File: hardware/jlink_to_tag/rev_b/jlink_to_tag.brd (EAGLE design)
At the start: 29.2 x 35.6 mm, 12 parts, among them J2 JLINK_6PIN_TAG-CON, U1 LT1763CS8-3.3

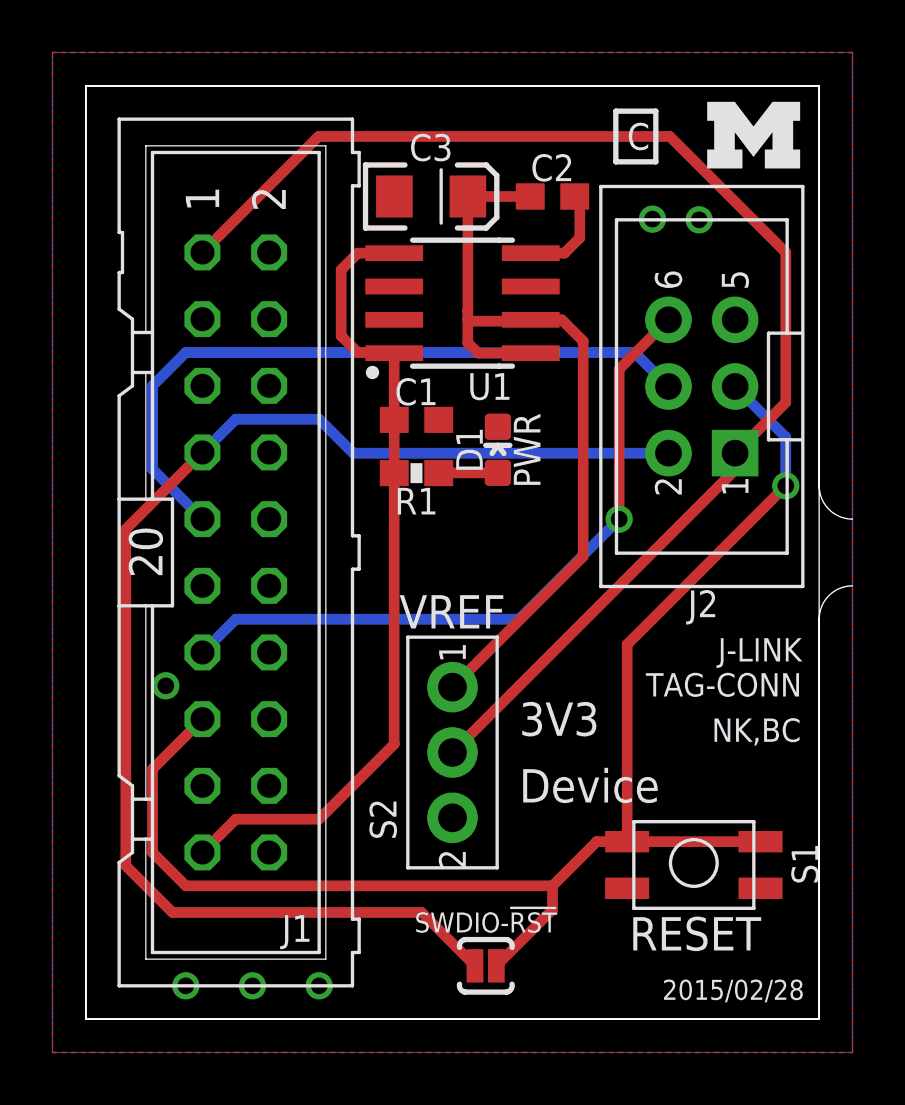
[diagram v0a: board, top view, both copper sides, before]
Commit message: revert rev b to the version that was fabbed
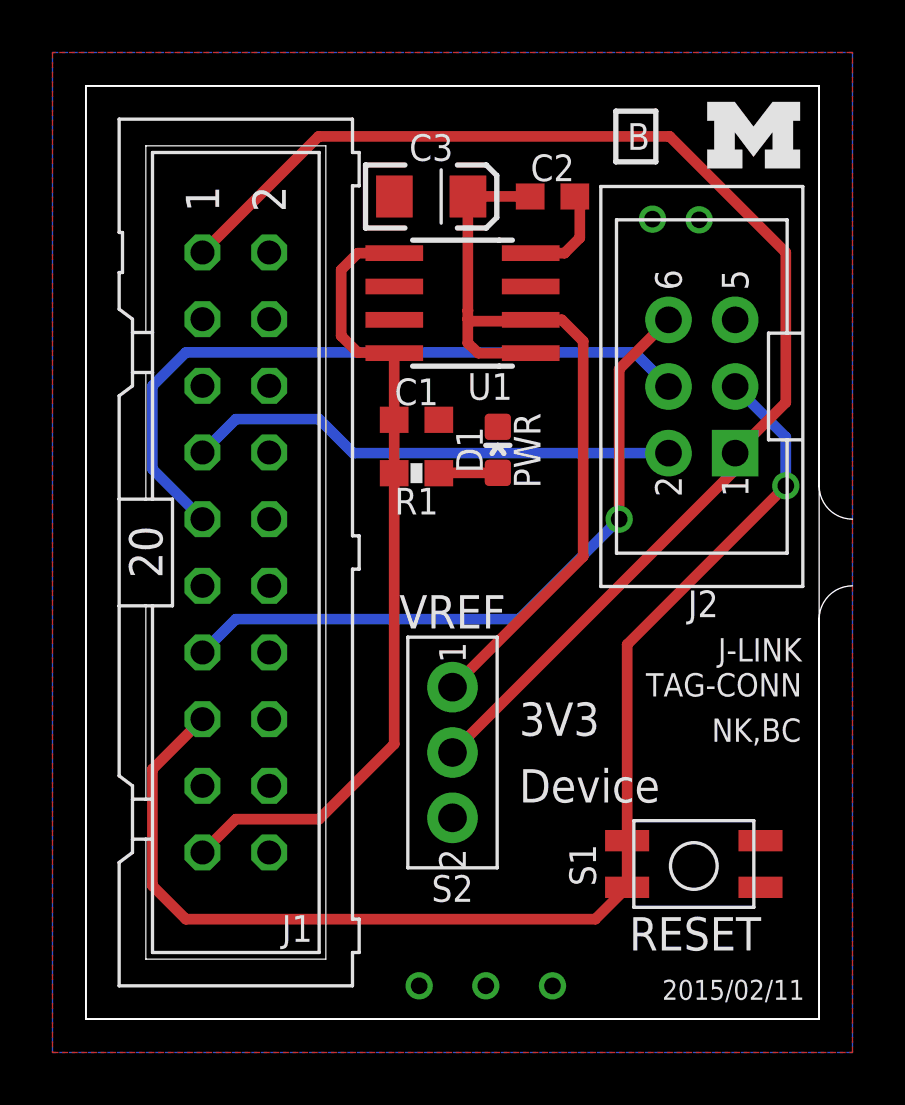
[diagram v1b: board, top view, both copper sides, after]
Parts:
- removed SJ1: SOLDERJUMPERNC2, SparkFun-Passives:SJ_2S-NOTRACE
- turned S1 to 0 degrees
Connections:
- net GND: now also S1.P$3; no longer S1.P$2
- net NRESET: now also S1.P$2; no longer S1.P$3, SJ1.1
- net SWDIO/TMS: no longer SJ1.2
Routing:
- net SWDIO/TMS: track 50.7 -> 18.8 mm
- net NRESET: track 54.8 -> 48.6 mm
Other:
- board text added: "2015/02/11"
- board text added: "B"
- board text removed: "2015/02/28"
- board text removed: "C"
- board text removed: "SWDIO-!RST"
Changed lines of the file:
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@@
 <setting verticaltext="up"/>
 </settings>
-<grid distance="10" unitdist="mil" unit="mil" style="lines" multiple="1" display="yes" altdistance="0.005" altunitdist="inch" altunit="inch"/>
+<grid distance="0.05" unitdist="inch" unit="inch" style="lines" multiple="1" display="yes" altdistance="0.005" altunitdist="inch" altunit="inch"/>
 <layers>
 <layer number="1" name="Top" color="4" fill="1" visible="yes" active="yes"/>
@@
 TAG-CONN</text>
 <text x="27.2542" y="10.5664" size="0.889" layer="21" font="vector" ratio="12" align="bottom-right">NK,BC</text>
-<text x="27.3812" y="0.7366" size="0.762" layer="21" font="vector" ratio="12" align="bottom-right">2015/02/28</text>
+<text x="27.3812" y="0.7366" size="0.762" layer="21" font="vector" ratio="12" align="bottom-right">2015/02/11</text>
 <text x="16.3068" y="21.6662" size="1.016" layer="21" ratio="12" rot="R90" align="top-center">PWR</text>
 <wire x1="0" y1="35.56" x2="0" y2="20.32" width="0" layer="151"/>
@@
 <text x="16.51" y="8.89" size="1.27" layer="21" font="vector" ratio="12" align="center-left">Device</text>
 <text x="13.97" y="14.8844" size="1.27" layer="21" font="vector" ratio="12" rot="R180" align="top-center">VREF</text>
-<text x="21.0566" y="33.6296" size="1.016" layer="21" font="vector" ratio="12" align="center">C</text>
+<text x="21.0566" y="33.6296" size="1.016" layer="21" font="vector" ratio="12" align="center">B</text>
 <wire x1="20.193" y1="32.6644" x2="21.717" y2="32.6644" width="0.2032" layer="21"/>
 <wire x1="21.717" y1="32.6644" x2="21.717" y2="34.5948" width="0.2032" layer="21"/>
 <wire x1="21.717" y1="34.5948" x2="20.193" y2="34.5948" width="0.2032" layer="21"/>
 <wire x1="20.193" y1="34.5948" x2="20.193" y2="32.6644" width="0.2032" layer="21"/>
-<text x="15.24" y="3.302" size="0.762" layer="21" font="vector" ratio="12" align="bottom-center">SWDIO-!RST</text>
-<circle x="10.922" y="24.638" radius="0.254" width="0" layer="21"/>
 </plain>
 <attributes>
@@
 <attribute name="VALUE" x="11.5824" y="19.6596" size="0.4064" layer="27" font="vector"/>
 </element>
-<element name="S1" library="switches" package="EVQP2" value="EVQP2" x="23.1648" y="5.8928" smashed="yes" rot="R180">
-<attribute name="DIGIKEY" value="P11084SCT-ND" x="23.1648" y="5.8928" size="1.778" layer="27" rot="R180" display="off"/>
-<attribute name="NAME" x="26.8922" y="5.9182" size="1.016" layer="25" font="vector" ratio="12" rot="R270" align="bottom-center"/>
-<attribute name="VALUE" x="26.4668" y="9.0488" size="1.27" layer="27" font="vector" ratio="10" rot="R180"/>
+<element name="S1" library="switches" package="EVQP2" value="EVQP2" x="23.1648" y="5.8928" smashed="yes">
+<attribute name="DIGIKEY" value="P11084SCT-ND" x="23.1648" y="5.8928" size="1.778" layer="27" display="off"/>
+<attribute name="NAME" x="19.4374" y="5.8674" size="1.016" layer="25" font="vector" ratio="12" rot="R90" align="bottom-center"/>
+<attribute name="VALUE" x="19.8628" y="2.7368" size="1.27" layer="27" font="vector" ratio="10"/>
 </element>
 <element name="S2" library="switches" package="TE_SSA12/SPDT" value="TE_SSA12/SPDT" x="13.97" y="10.16" smashed="yes" rot="R270">
 <attribute name="DIGIKEY" value="450-1602-ND" x="13.97" y="10.16" size="1.778" layer="27" rot="R270" display="off"/>
-<attribute name="NAME" x="11.8364" y="7.62" size="1.016" layer="25" font="vector" ratio="12" rot="R90" align="bottom-center"/>
+<attribute name="NAME" x="13.97" y="5.4864" size="1.016" layer="25" font="vector" ratio="12" rot="R180" align="bottom-center"/>
 <attribute name="VALUE" x="10.795" y="10.16" size="1.016" layer="27" font="vector" ratio="12" rot="R270" align="bottom-center"/>
-</element>
-<element name="SJ1" library="SparkFun-Passives" package="SJ_2S-NOTRACE" value="SOLDERJUMPERNC2" x="15.24" y="2.032" smashed="yes" rot="R180">
-<attribute name="VALUE" x="16.1925" y="3.683" size="0.4064" layer="27" rot="R180"/>
 </element>
 </elements>
@@
 <vertex x="-1.27" y="-1.27"/>
 </polygon>
-<contactref element="S1" pad="P$2"/>
+<contactref element="S1" pad="P$3"/>
 <contactref element="S1" pad="P$4"/>
-<via x="3.81" y="1.27" extent="1-16" drill="0.635"/>
-<via x="6.35" y="1.27" extent="1-16" drill="0.635"/>
-<via x="8.89" y="1.27" extent="1-16" drill="0.635"/>
+<via x="12.7" y="1.27" extent="1-16" drill="0.635"/>
+<via x="15.24" y="1.27" extent="1-16" drill="0.635"/>
+<via x="17.78" y="1.27" extent="1-16" drill="0.635"/>
 <via x="21.59" y="30.48" extent="1-16" drill="0.635"/>
 <via x="23.368" y="30.4546" extent="1-16" drill="0.635"/>
-<via x="3.048" y="12.7" extent="1-16" drill="0.635"/>
 </signal>
 <signal name="NRESET">
@@
 <contactref element="J2" pad="3"/>
 <contactref element="S1" pad="P$1"/>
-<contactref element="S1" pad="P$3"/>
+<contactref element="S1" pad="P$2"/>
 <wire x1="4.445" y1="11.43" x2="2.54" y2="9.525" width="0.4064" layer="1"/>
-<wire x1="25.7048" y1="6.7628" x2="20.6248" y2="6.7628" width="0.4064" layer="1"/>
+<wire x1="2.54" y1="9.525" x2="2.54" y2="5.08" width="0.4064" layer="1"/>
+<wire x1="2.54" y1="5.08" x2="3.81" y2="3.81" width="0.4064" layer="1"/>
+<wire x1="20.6248" y1="5.0228" x2="20.6248" y2="6.8008" width="0.4064" layer="1"/>
 <via x="26.67" y="20.32" extent="1-16" drill="0.635"/>
 <wire x1="26.67" y1="20.32" x2="26.67" y2="22.1742" width="0.4064" layer="16"/>
 <wire x1="26.67" y1="22.1742" x2="24.7396" y2="24.1046" width="0.4064" layer="16"/>
-<wire x1="20.6248" y1="6.7628" x2="20.6248" y2="14.2748" width="0.4064" layer="1"/>
+<wire x1="3.81" y1="3.81" x2="19.412" y2="3.81" width="0.4064" layer="1"/>
+<wire x1="19.412" y1="3.81" x2="20.6248" y2="5.0228" width="0.4064" layer="1"/>
+<wire x1="20.6248" y1="6.8008" x2="20.6248" y2="14.2748" width="0.4064" layer="1"/>
 <wire x1="20.6248" y1="14.2748" x2="26.67" y2="20.32" width="0.4064" layer="1"/>
-<contactref element="SJ1" pad="1"/>
-<wire x1="2.54" y1="9.525" x2="2.54" y2="6.35" width="0.4064" layer="1"/>
-<wire x1="2.54" y1="6.35" x2="3.81" y2="5.08" width="0.4064" layer="1"/>
-<wire x1="3.81" y1="5.08" x2="17.78" y2="5.08" width="0.4064" layer="1"/>
-<wire x1="17.78" y1="5.08" x2="19.4628" y2="6.7628" width="0.4064" layer="1"/>
-<wire x1="19.4628" y1="6.7628" x2="20.6248" y2="6.7628" width="0.4064" layer="1"/>
-<wire x1="15.6409" y1="2.032" x2="17.78" y2="4.1711" width="0.4064" layer="1"/>
-<wire x1="17.78" y1="4.1711" x2="17.78" y2="5.08" width="0.4064" layer="1"/>
 </signal>
 <signal name="SWCLK/TCK">
@@
 <wire x1="5.715" y1="22.86" x2="8.89" y2="22.86" width="0.4064" layer="16"/>
 <wire x1="8.89" y1="22.86" x2="10.1854" y2="21.5646" width="0.4064" layer="16"/>
-<contactref element="SJ1" pad="2"/>
-<wire x1="4.445" y1="21.59" x2="1.524" y2="18.669" width="0.4064" layer="1"/>
-<wire x1="1.524" y1="18.669" x2="1.524" y2="5.842" width="0.4064" layer="1"/>
-<wire x1="1.524" y1="5.842" x2="3.302" y2="4.064" width="0.4064" layer="1"/>
-<wire x1="3.302" y1="4.064" x2="12.7953" y2="4.064" width="0.4064" layer="1"/>
-<wire x1="12.7953" y1="4.064" x2="14.8273" y2="2.032" width="0.4064" layer="1"/>
 </signal>
 <signal name="SWO/TDO">

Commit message: bug fixes to rev b
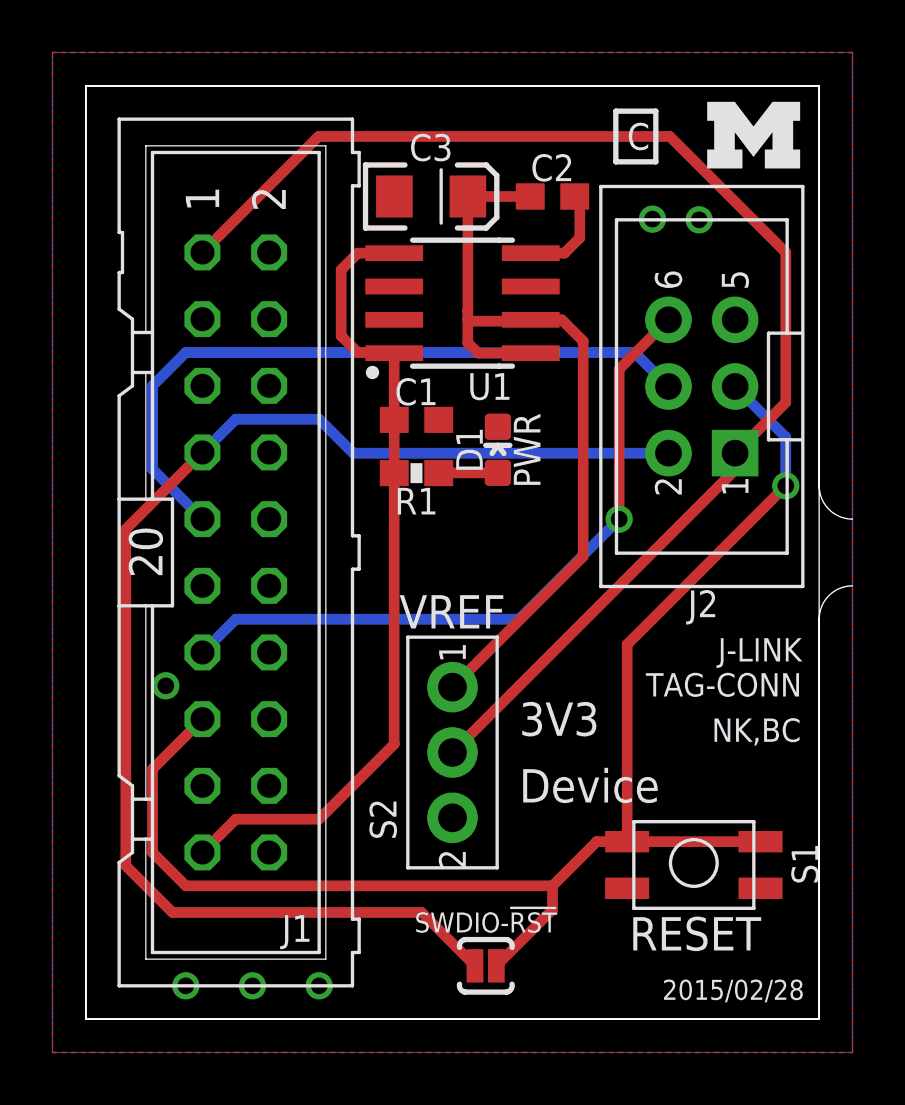
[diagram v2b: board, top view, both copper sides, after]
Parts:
- added SJ1: SOLDERJUMPERNC2, SparkFun-Passives:SJ_2S-NOTRACE
- turned S1 to 180 degrees
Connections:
- net GND: now also S1.P$2; no longer S1.P$3
- net NRESET: now also S1.P$3, SJ1.1; no longer S1.P$2
- net SWDIO/TMS: now also SJ1.2
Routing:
- net SWDIO/TMS: track 18.8 -> 50.7 mm
- net NRESET: track 48.6 -> 54.8 mm
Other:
- board text added: "2015/02/28"
- board text added: "C"
- board text added: "SWDIO-!RST"
- board text removed: "2015/02/11"
- board text removed: "B"
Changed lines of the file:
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@@
 <setting verticaltext="up"/>
 </settings>
-<grid distance="0.05" unitdist="inch" unit="inch" style="lines" multiple="1" display="yes" altdistance="0.005" altunitdist="inch" altunit="inch"/>
+<grid distance="10" unitdist="mil" unit="mil" style="lines" multiple="1" display="yes" altdistance="0.005" altunitdist="inch" altunit="inch"/>
 <layers>
 <layer number="1" name="Top" color="4" fill="1" visible="yes" active="yes"/>
@@
 TAG-CONN</text>
 <text x="27.2542" y="10.5664" size="0.889" layer="21" font="vector" ratio="12" align="bottom-right">NK,BC</text>
-<text x="27.3812" y="0.7366" size="0.762" layer="21" font="vector" ratio="12" align="bottom-right">2015/02/11</text>
+<text x="27.3812" y="0.7366" size="0.762" layer="21" font="vector" ratio="12" align="bottom-right">2015/02/28</text>
 <text x="16.3068" y="21.6662" size="1.016" layer="21" ratio="12" rot="R90" align="top-center">PWR</text>
 <wire x1="0" y1="35.56" x2="0" y2="20.32" width="0" layer="151"/>
@@
 <text x="16.51" y="8.89" size="1.27" layer="21" font="vector" ratio="12" align="center-left">Device</text>
 <text x="13.97" y="14.8844" size="1.27" layer="21" font="vector" ratio="12" rot="R180" align="top-center">VREF</text>
-<text x="21.0566" y="33.6296" size="1.016" layer="21" font="vector" ratio="12" align="center">B</text>
+<text x="21.0566" y="33.6296" size="1.016" layer="21" font="vector" ratio="12" align="center">C</text>
 <wire x1="20.193" y1="32.6644" x2="21.717" y2="32.6644" width="0.2032" layer="21"/>
 <wire x1="21.717" y1="32.6644" x2="21.717" y2="34.5948" width="0.2032" layer="21"/>
 <wire x1="21.717" y1="34.5948" x2="20.193" y2="34.5948" width="0.2032" layer="21"/>
 <wire x1="20.193" y1="34.5948" x2="20.193" y2="32.6644" width="0.2032" layer="21"/>
+<text x="15.24" y="3.302" size="0.762" layer="21" font="vector" ratio="12" align="bottom-center">SWDIO-!RST</text>
+<circle x="10.922" y="24.638" radius="0.254" width="0" layer="21"/>
 </plain>
 <attributes>
@@
 <attribute name="VALUE" x="11.5824" y="19.6596" size="0.4064" layer="27" font="vector"/>
 </element>
-<element name="S1" library="switches" package="EVQP2" value="EVQP2" x="23.1648" y="5.8928" smashed="yes">
-<attribute name="DIGIKEY" value="P11084SCT-ND" x="23.1648" y="5.8928" size="1.778" layer="27" display="off"/>
-<attribute name="NAME" x="19.4374" y="5.8674" size="1.016" layer="25" font="vector" ratio="12" rot="R90" align="bottom-center"/>
-<attribute name="VALUE" x="19.8628" y="2.7368" size="1.27" layer="27" font="vector" ratio="10"/>
+<element name="S1" library="switches" package="EVQP2" value="EVQP2" x="23.1648" y="5.8928" smashed="yes" rot="R180">
+<attribute name="DIGIKEY" value="P11084SCT-ND" x="23.1648" y="5.8928" size="1.778" layer="27" rot="R180" display="off"/>
+<attribute name="NAME" x="26.8922" y="5.9182" size="1.016" layer="25" font="vector" ratio="12" rot="R270" align="bottom-center"/>
+<attribute name="VALUE" x="26.4668" y="9.0488" size="1.27" layer="27" font="vector" ratio="10" rot="R180"/>
 </element>
 <element name="S2" library="switches" package="TE_SSA12/SPDT" value="TE_SSA12/SPDT" x="13.97" y="10.16" smashed="yes" rot="R270">
 <attribute name="DIGIKEY" value="450-1602-ND" x="13.97" y="10.16" size="1.778" layer="27" rot="R270" display="off"/>
-<attribute name="NAME" x="13.97" y="5.4864" size="1.016" layer="25" font="vector" ratio="12" rot="R180" align="bottom-center"/>
+<attribute name="NAME" x="11.8364" y="7.62" size="1.016" layer="25" font="vector" ratio="12" rot="R90" align="bottom-center"/>
 <attribute name="VALUE" x="10.795" y="10.16" size="1.016" layer="27" font="vector" ratio="12" rot="R270" align="bottom-center"/>
+</element>
+<element name="SJ1" library="SparkFun-Passives" package="SJ_2S-NOTRACE" value="SOLDERJUMPERNC2" x="15.24" y="2.032" smashed="yes" rot="R180">
+<attribute name="VALUE" x="16.1925" y="3.683" size="0.4064" layer="27" rot="R180"/>
 </element>
 </elements>
@@
 <vertex x="-1.27" y="-1.27"/>
 </polygon>
-<contactref element="S1" pad="P$3"/>
+<contactref element="S1" pad="P$2"/>
 <contactref element="S1" pad="P$4"/>
-<via x="12.7" y="1.27" extent="1-16" drill="0.635"/>
-<via x="15.24" y="1.27" extent="1-16" drill="0.635"/>
-<via x="17.78" y="1.27" extent="1-16" drill="0.635"/>
+<via x="3.81" y="1.27" extent="1-16" drill="0.635"/>
+<via x="6.35" y="1.27" extent="1-16" drill="0.635"/>
+<via x="8.89" y="1.27" extent="1-16" drill="0.635"/>
 <via x="21.59" y="30.48" extent="1-16" drill="0.635"/>
 <via x="23.368" y="30.4546" extent="1-16" drill="0.635"/>
+<via x="3.048" y="12.7" extent="1-16" drill="0.635"/>
 </signal>
 <signal name="NRESET">
@@
 <contactref element="J2" pad="3"/>
 <contactref element="S1" pad="P$1"/>
-<contactref element="S1" pad="P$2"/>
+<contactref element="S1" pad="P$3"/>
 <wire x1="4.445" y1="11.43" x2="2.54" y2="9.525" width="0.4064" layer="1"/>
-<wire x1="2.54" y1="9.525" x2="2.54" y2="5.08" width="0.4064" layer="1"/>
-<wire x1="2.54" y1="5.08" x2="3.81" y2="3.81" width="0.4064" layer="1"/>
-<wire x1="20.6248" y1="5.0228" x2="20.6248" y2="6.8008" width="0.4064" layer="1"/>
+<wire x1="25.7048" y1="6.7628" x2="20.6248" y2="6.7628" width="0.4064" layer="1"/>
 <via x="26.67" y="20.32" extent="1-16" drill="0.635"/>
 <wire x1="26.67" y1="20.32" x2="26.67" y2="22.1742" width="0.4064" layer="16"/>
 <wire x1="26.67" y1="22.1742" x2="24.7396" y2="24.1046" width="0.4064" layer="16"/>
-<wire x1="3.81" y1="3.81" x2="19.412" y2="3.81" width="0.4064" layer="1"/>
-<wire x1="19.412" y1="3.81" x2="20.6248" y2="5.0228" width="0.4064" layer="1"/>
-<wire x1="20.6248" y1="6.8008" x2="20.6248" y2="14.2748" width="0.4064" layer="1"/>
+<wire x1="20.6248" y1="6.7628" x2="20.6248" y2="14.2748" width="0.4064" layer="1"/>
 <wire x1="20.6248" y1="14.2748" x2="26.67" y2="20.32" width="0.4064" layer="1"/>
+<contactref element="SJ1" pad="1"/>
+<wire x1="2.54" y1="9.525" x2="2.54" y2="6.35" width="0.4064" layer="1"/>
+<wire x1="2.54" y1="6.35" x2="3.81" y2="5.08" width="0.4064" layer="1"/>
+<wire x1="3.81" y1="5.08" x2="17.78" y2="5.08" width="0.4064" layer="1"/>
+<wire x1="17.78" y1="5.08" x2="19.4628" y2="6.7628" width="0.4064" layer="1"/>
+<wire x1="19.4628" y1="6.7628" x2="20.6248" y2="6.7628" width="0.4064" layer="1"/>
+<wire x1="15.6409" y1="2.032" x2="17.78" y2="4.1711" width="0.4064" layer="1"/>
+<wire x1="17.78" y1="4.1711" x2="17.78" y2="5.08" width="0.4064" layer="1"/>
 </signal>
 <signal name="SWCLK/TCK">
@@
 <wire x1="5.715" y1="22.86" x2="8.89" y2="22.86" width="0.4064" layer="16"/>
 <wire x1="8.89" y1="22.86" x2="10.1854" y2="21.5646" width="0.4064" layer="16"/>
+<contactref element="SJ1" pad="2"/>
+<wire x1="4.445" y1="21.59" x2="1.524" y2="18.669" width="0.4064" layer="1"/>
+<wire x1="1.524" y1="18.669" x2="1.524" y2="5.842" width="0.4064" layer="1"/>
+<wire x1="1.524" y1="5.842" x2="3.302" y2="4.064" width="0.4064" layer="1"/>
+<wire x1="3.302" y1="4.064" x2="12.7953" y2="4.064" width="0.4064" layer="1"/>
+<wire x1="12.7953" y1="4.064" x2="14.8273" y2="2.032" width="0.4064" layer="1"/>
 </signal>
 <signal name="SWO/TDO">
